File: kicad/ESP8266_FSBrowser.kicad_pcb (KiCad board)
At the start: 2 copper layers, 19 parts, among them P1 POWER, P2 ADC, P3 SERIAL, P4 GPIO, SW1 RESET, SW2 AP_ENABLE, SW3 FLASH, U1 ESP-12E, U2 LM1117-3.3

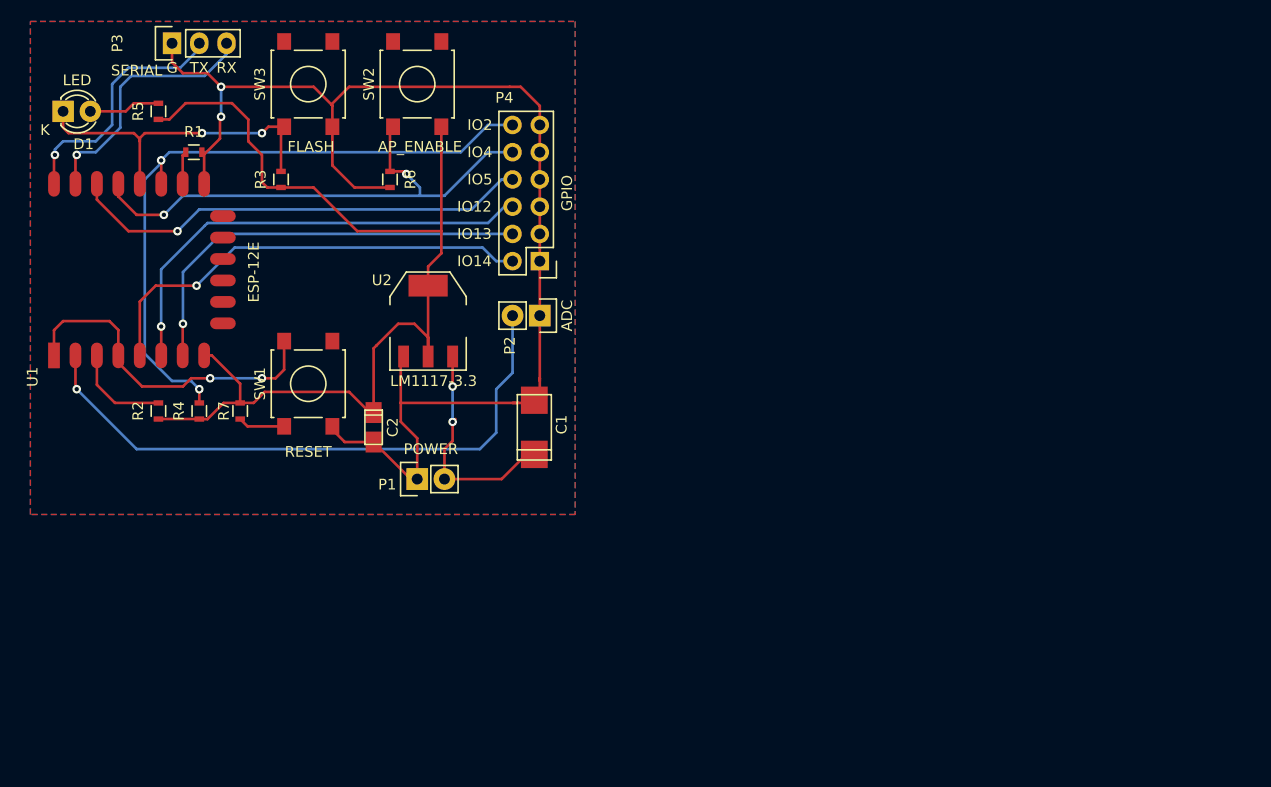
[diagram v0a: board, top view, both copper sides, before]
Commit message: Play with kicad files
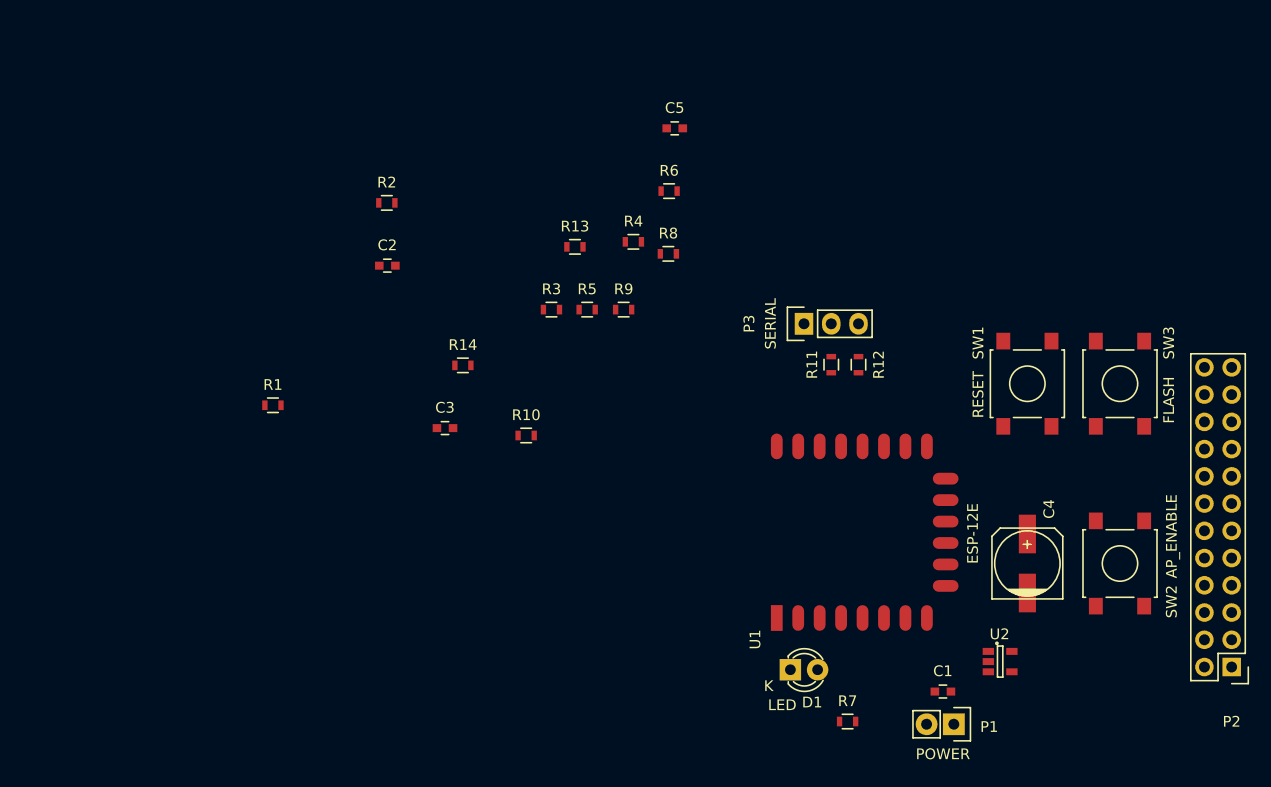
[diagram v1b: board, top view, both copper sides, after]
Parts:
- removed P4: GPIO, Pin_Headers:Pin_Header_Straight_2x06
- added C3: 470p, Capacitors_SMD:C_0603, F.Cu at (94.0, 71.4)
- added C4: 100u, Capacitors_SMD:c_elec_6.3x5.8, F.Cu at (148.3, 84.1)
- added C5: 470p, Capacitors_SMD:C_0603, F.Cu at (115.5, 43.5)
- added R10: 0, Resistors_SMD:R_0603, F.Cu at (101.6, 72.1)
- added R11: 470, Resistors_SMD:R_0603, F.Cu at (130.0, 65.5)
- added R12: 470, Resistors_SMD:R_0603, F.Cu at (132.6, 65.5)
- added R13: 220k(1%), Resistors_SMD:R_0603, F.Cu at (106.1, 54.5)
- added R14: 100k(1%), Resistors_SMD:R_0603, F.Cu at (95.7, 65.6)
- added R8: 10k, Resistors_SMD:R_0603, F.Cu at (114.9, 55.2)
- added R9: 220, Resistors_SMD:R_0603, F.Cu at (110.7, 60.4)
- C1: value 10u -> 1u; footprint Capacitors_Tantalum_SMD:TantalC_SizeU_EIA-6032 -> Capacitors_SMD:C_0603
- C2: value 1u -> 10u; footprint Capacitors_Tantalum_SMD:TantalC_SizeS_EIA-3216 -> Capacitors_SMD:C_0603
- P2: value ADC -> GPIO; footprint Pin_Headers:Pin_Header_Straight_1x02 -> Pin_Headers:Pin_Header_Straight_2x12
- R5: value 330 -> 470
- U2: value LM1117-3.3 -> SPX3819M5-L-3-3; footprint TO_SOT_Packages_SMD:SOT-223 -> TO_SOT_Packages_SMD:SOT-23-5
- moved D1 85.5 mm to (126.2, 94.0)
- moved SW3 80.7 mm to (157.0, 67.3)
- moved SW2 79.3 mm to (157.0, 84.1), turned to 270 degrees
- moved P2 72.4 mm to (167.4, 93.7), turned to 180 degrees
- moved U1 71.7 mm to (125.0, 89.2)
- moved SW1 67.1 mm to (148.3, 67.3), turned to 270 degrees
- moved P3 64.5 mm to (127.5, 61.7)
- moved R7 63.6 mm to (131.6, 98.8), turned to 0 degrees
- moved U2 62.1 mm to (145.8, 93.2)
- moved P1 55.0 mm to (141.5, 99.1), turned to 270 degrees
- moved C1 45.4 mm to (140.5, 96.0), turned to 0 degrees
- moved R5 44.0 mm to (107.3, 60.4), turned to 0 degrees
- moved R4 43.4 mm to (111.6, 54.1), turned to 0 degrees
- moved R2 28.8 mm to (88.6, 50.4), turned to 0 degrees
- moved R3 28.0 mm to (104.0, 60.4), turned to 0 degrees
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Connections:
- net Net-(R1-Pad1) renamed GPIO15
- C1 pad 1: Net-(C1-Pad1) -> +5V
- D1 pad 1: Net-(D1-Pad1) -> GPIO16
- P1 pad 2: Net-(C1-Pad1) -> +5V
- P2 pad 2: ADC -> Net-(P2-Pad2)
- R2 pad 1: +3V3 -> CH_PD
- R2 pad 2: Net-(R2-Pad2) -> +3V3
- R3 pad 1: +3V3 -> GPIO2
- R3 pad 2: Net-(D1-Pad1) -> +3V3
- R4 pad 1: +3V3 -> GPIO0
- R4 pad 2: GPIO2 -> +3V3
- R6 pad 1: AP_EN -> GPIO4
- R7 pad 1: +3V3 -> GPIO16
- R7 pad 2: RST -> Net-(R10-Pad2)
- SW1 pad 1: RST -> GND
- SW1 pad 2: GND -> Net-(R10-Pad2)
- SW2 pad 1: AP_EN -> GPIO4
- SW3 pad 1: Net-(D1-Pad1) -> Net-(R9-Pad1)
- U1 pad 18: Net-(D1-Pad1) -> GPIO0
- U1 pad 19: AP_EN -> GPIO4
- U1 pad 21: Net-(P3-Pad3) -> Net-(R12-Pad2)
- U1 pad 22: Net-(P3-Pad2) -> Net-(R11-Pad2)
- U1 pad 3: Net-(R2-Pad2) -> CH_PD
- U1 pad 4: RST -> GPIO16
- U2 pad 1: GND -> +5V
- U2 pad 2: +3V3 -> GND
- U2 pad 3: Net-(C1-Pad1) -> +5V
- U2 pad 4: +3V3 -> Net-(C5-Pad1)
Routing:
- net GND: track 124.1 -> 0.00 mm, vias 2 -> 0
- net +3V3: track 99.1 -> 0.00 mm
- net GPIO2: track 62.7 -> 0.00 mm, vias 2 -> 0
- net ADC: track 56.8 -> 0.00 mm, vias 1 -> 0
- net AP_EN: track 49.5 -> 0.00 mm, vias 2 -> 0
- net GPIO5: track 43.4 -> 0.00 mm, vias 1 -> 0
- net GPIO12: track 43.2 -> 0.00 mm, vias 1 -> 0
- net GPIO14: track 42.6 -> 0.00 mm, vias 1 -> 0
- net GPIO13: track 40.0 -> 0.00 mm, vias 1 -> 0
- net RST: track 36.2 -> 0.00 mm, vias 2 -> 0
- net Net-(D1-Pad1): track 31.8 -> 0.00 mm, vias 2 -> 0
- net Net-(P3-Pad3): track 23.9 -> 0.00 mm, vias 1 -> 0
- net Net-(P3-Pad2): track 23.3 -> 0.00 mm, vias 1 -> 0
- net Net-(C1-Pad1): track 21.5 -> 0.00 mm, vias 2 -> 0
- net Net-(R2-Pad2): track 9.18 -> 0.00 mm
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- removed copper zone on B.Cu, net GND
- removed copper zone on F.Cu, net GND
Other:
- board text removed: "G"
- board text removed: "IO12"
- board text removed: "IO13"
- board text removed: "IO14"
- board text removed: "IO2"
- board text removed: "IO4"
- board text removed: "IO5"
- board text removed: "RX"
- board text removed: "TX"
